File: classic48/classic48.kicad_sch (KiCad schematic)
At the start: 75 parts, among them SW1 Switch, SW10 Switch, SW11 Switch, SW12 Switch, SW13 Switch, SW14 Switch, SW15 Switch, SW16 Switch, SW17 Switch, SW18 Switch, SW19 Switch, SW2 Switch, SW20 Switch, SW21 Switch, SW22 Switch, SW23 Switch, SW24 Switch, SW3 Switch, SW4 Switch, SW5 Switch, SW6 Switch, SW7 Switch, SW8 Switch, SW9 Switch, U1 RP2040_Pro_Micro, U2 TRRS

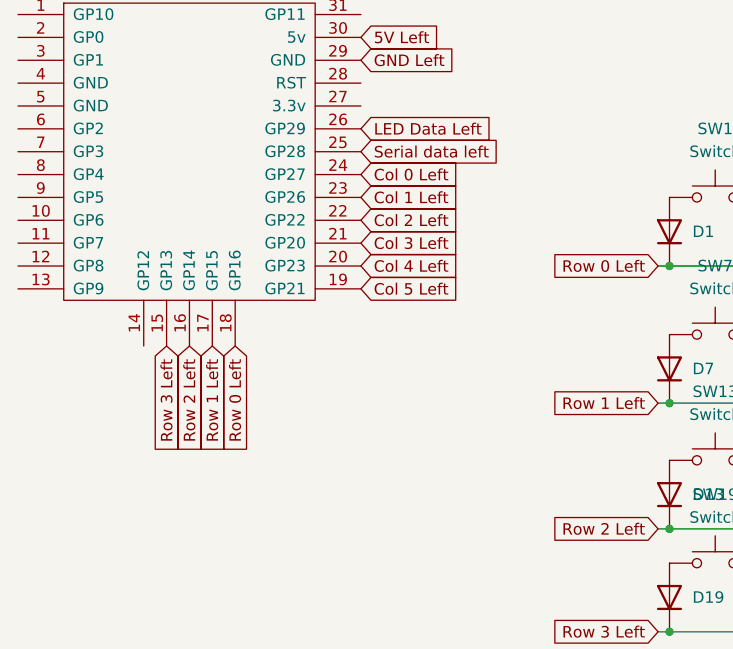
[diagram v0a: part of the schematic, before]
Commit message: feat: finish tracks
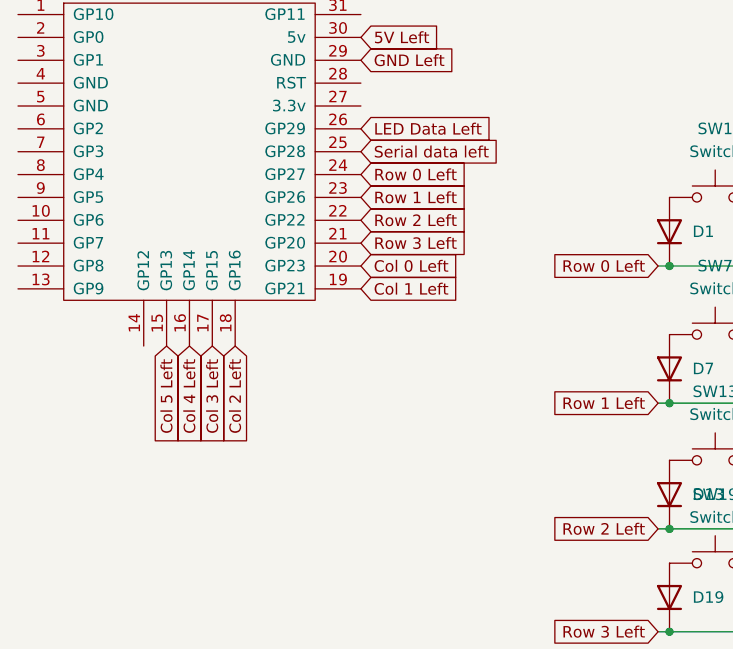
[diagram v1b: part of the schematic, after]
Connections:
- net Col 0 Left: now also U1.20 (GP23); no longer U1.24 (GP27)
- net Col 1 Left: now also U1.19 (GP21); no longer U1.23 (GP26)
- net Col 2 Left: now also U1.18 (GP16); no longer U1.22 (GP22)
- net Col 3 Left: now also U1.17 (GP15); no longer U1.21 (GP20)
- net Col 4 Left: now also U1.16 (GP14); no longer U1.20 (GP23)
- net Col 5 Left: now also U1.15 (GP13); no longer U1.19 (GP21)
- net Row 0 Left: now also U1.24 (GP27); no longer U1.18 (GP16)
- net Row 1 Left: now also U1.23 (GP26); no longer U1.17 (GP15)
- net Row 2 Left: now also U1.22 (GP22); no longer U1.16 (GP14)
- net Row 3 Left: now also U1.21 (GP20); no longer U1.15 (GP13)
